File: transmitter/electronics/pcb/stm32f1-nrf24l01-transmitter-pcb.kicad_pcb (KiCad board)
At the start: 2 copper layers, 100 x 48 mm, 72 parts, among them J1 PA1/A1, J10 PB3, J11 PB4, J12 PB5, J13 PB6, J14 PB7, J15 PB8, J16 PB10, J17 PB11, J18 External charger LED, J19 BATTERY, J2 PA2/A2, J20 Red, J21 Blue, J22 POWER SWITCH, J23 USB, J24 UART, J25 SWD, J26 Buzzer, J27 NRF24 connector, J29 Meter, J3 PA3/A3, J30 LED, J4 PA4/A4, J5 PA5/A5, J6 PA6/A6, J7 PA7/A7, J8 PB0/A8, J9 PB1/A9, Q1 PMV30UN, SW1 RESET, U1 MCP1703A-3302, U2 LIPO_CHARGER_+_PROTECTION, U3 STM32F103CBT6, U4 MCP1703A-3302, Y1 8MHz

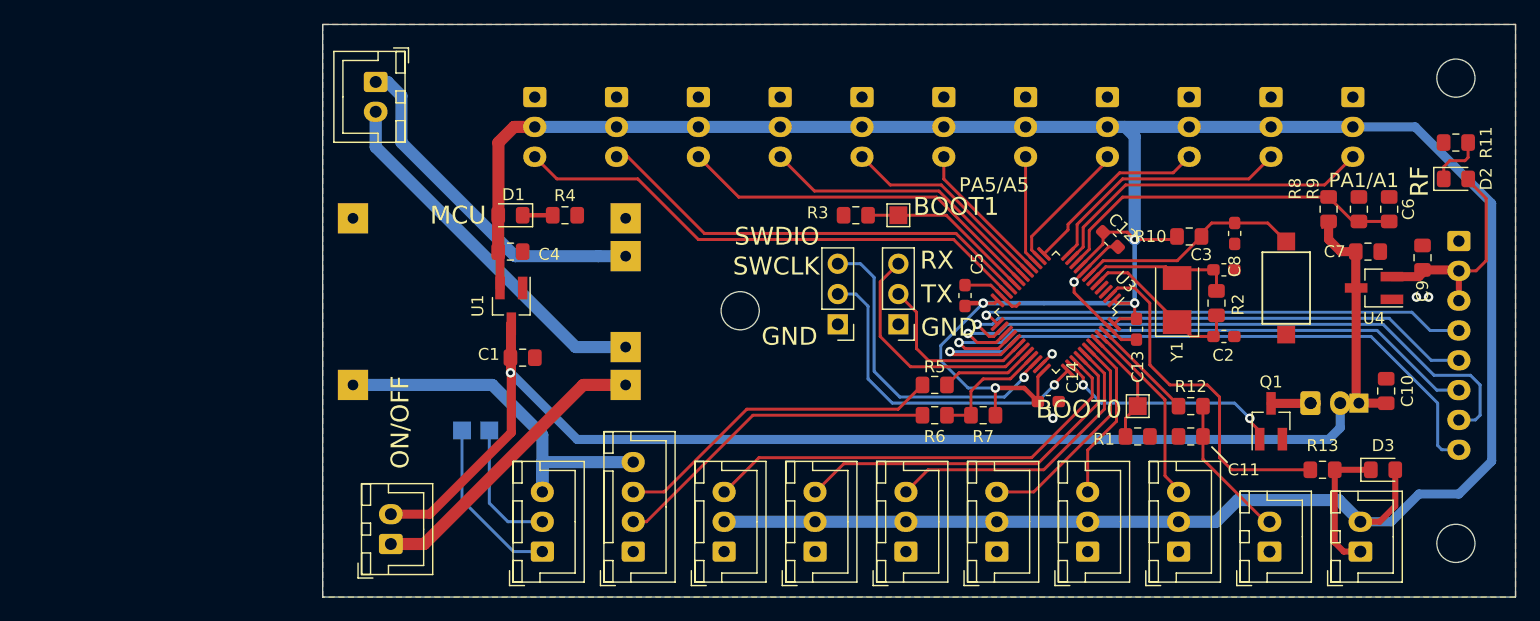
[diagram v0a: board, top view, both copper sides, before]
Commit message: Make combined PCB
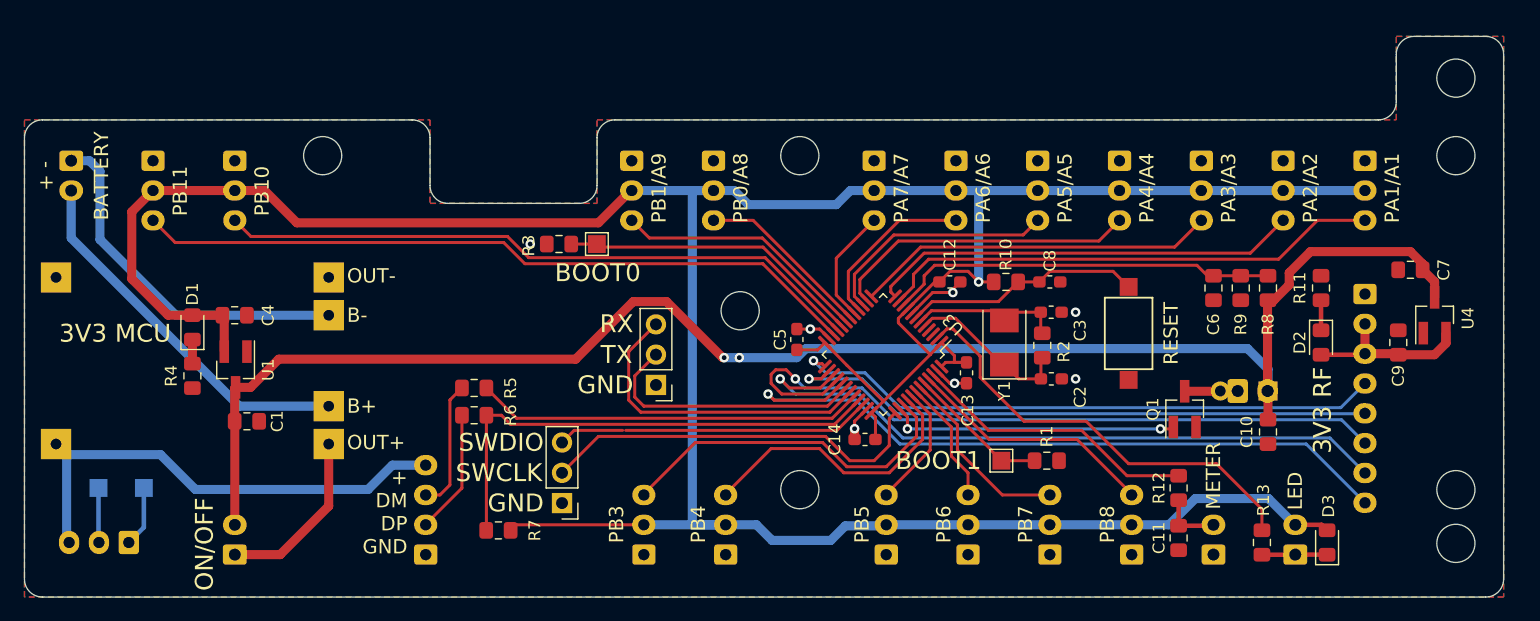
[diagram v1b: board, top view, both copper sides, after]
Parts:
- added H4: MountingHole, MountingHole:MountingHole_3.2mm_M3_DIN965, F.Cu at (140.0, 91.0)
- added H5: MountingHole, MountingHole:MountingHole_3.2mm_M3_DIN965, F.Cu at (140.0, 63.0)
- added H6: MountingHole, MountingHole:MountingHole_3.2mm_M3_DIN965, F.Cu at (195.0, 63.0)
- added H7: MountingHole, MountingHole:MountingHole_3.2mm_M3_DIN965, F.Cu at (195.0, 91.0)
- added H8: MountingHole, MountingHole:MountingHole_3.2mm_M3_DIN965, F.Cu at (100.0, 63.0)
- J10, J11, J12, J13, J14, J15, J18, J19, J22, J23, J29, J30: moved to B.Cu
- moved R7 41.8 mm to (114.7, 94.4)
- moved R5 38.6 mm to (112.7, 82.5)
- moved R6 38.6 mm to (112.7, 84.8)
- moved J18 34.7 mm to (83.7, 95.4), turned to 180 degrees
- moved R4 34.0 mm to (89.1, 81.5), turned to 270 degrees
- moved J20 33.1 mm to (81.2, 90.9)
- moved J16 32.4 mm to (92.6, 63.4)
- moved J17 32.4 mm to (85.8, 63.4)
- moved D1 28.3 mm to (89.1, 77.4), turned to 90 degrees
- moved J25 27.5 mm to (120.1, 92.1)
- moved J21 27.1 mm to (85.0, 90.9)
- moved J19 26.4 mm to (78.9, 63.4)
- moved TP2 25.4 mm to (123.0, 70.4), turned to 90 degrees
- moved U2 25.4 mm to (89.1, 80.2)
- moved R3 25.0 mm to (119.8, 70.4)
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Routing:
- net /USBDP: track 10.3 -> 42.0 mm
- net /USBDM: track 7.81 -> 32.7 mm
- net Net-(J23-Pad2): track 27.9 -> 10.4 mm
- net Net-(J23-Pad3): track 28.0 -> 10.9 mm
- net /PB11: track 44.2 -> 61.0 mm
- net /PB10: track 37.5 -> 54.3 mm
- net /METER: track 8.69 -> 24.1 mm
- net /PA2-ADC2: track 21.4 -> 36.2 mm
- net +3V3: track 263.9 -> 278.7 mm, vias 4 -> 1
- net /PA3-ADC3: track 15.8 -> 30.3 mm
- net /PA4-ADC4: track 11.4 -> 25.8 mm
- net /PB5: track 24.8 -> 10.4 mm
- net /PA1-ADC1: track 28.0 -> 42.4 mm
- net VDD: track 122.1 -> 134.8 mm, vias 1 -> 2
- net /PA5-ADC5: track 9.20 -> 20.1 mm
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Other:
- board size 100 x 48 mm -> 124 x 47 mm
- net class Default: clearance 0.2 -> 0.2032; trace_width 0.25 -> 0.254
- rule trace_clearance: 0.2 -> 0.2032
- rule trace_min: 0.2 -> 0.2032
- board text added: "+ DM DP GND"
- board text added: "- +"
- board text added: "3V3 MCU"
- board text added: "3V3 RF"
- board text added: "B+"
- board text added: "B-"
- board text added: "BAT"
- board text added: "BATTERY"
- board text added: "BUZZER"
- board text added: "CHARGER LED"
- board text added: "LED"
- board text added: "METER"
- board text added: "NRF24L01P"
- board text added: "OUT+"
- board text added: "OUT-"
- board text added: "PA2/A2"
- board text added: "PA3/A3"
- board text added: "PA4/A4"
- board text added: "PA6/A6"
- board text added: "PA7/A7"
- board text added: "PB0/A8"
- board text added: "PB1/A9"
- board text added: "PB10"
- board text added: "PB11"
- board text added: "PB3"
- board text added: "PB4"
- board text added: "PB5"
- board text added: "PB6"
- board text added: "PB7"
- board text added: "PB8"
- board text added: "RESET"
- board text added: "USB"
- board text removed: "MCU"
- board text removed: "RF"
